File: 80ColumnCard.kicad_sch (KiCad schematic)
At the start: 37 parts, among them J1 Apple II Expansion Bus, J2 VIDEO & LIGHT PEN, Q1 2N3904, U1 74LS86, U14 74LS157, U15 74LS157, U16 74LS157, U18 74LS273, U19 MC6845, U2 74LS02, U21 74LS166, U22 74LS175, U23 74LS161, U3 2758{slash}16{slash}32, U4 74LS04, U5 74LS245, U6 74LS00, U7 4013, U8 4013, U9 74LS139, X6 CHAR INV, X7 SCREEN INV, Y1 17.430 MHZ

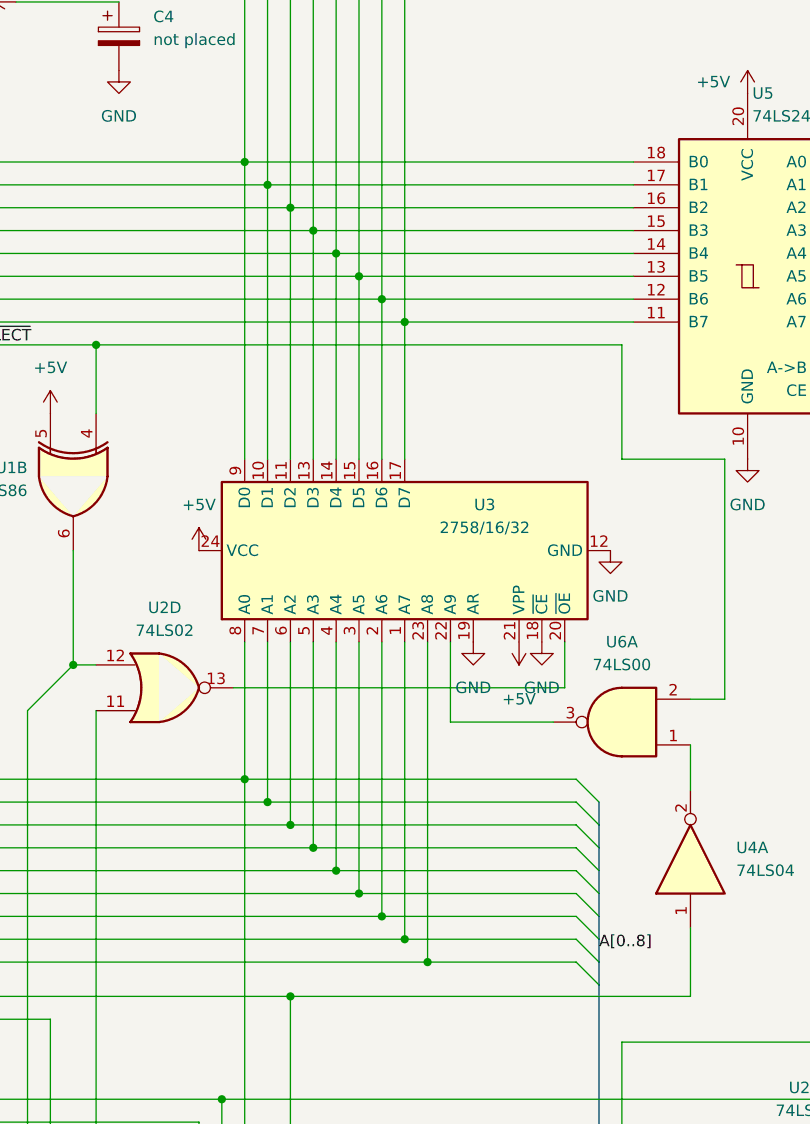
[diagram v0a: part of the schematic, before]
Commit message: updates
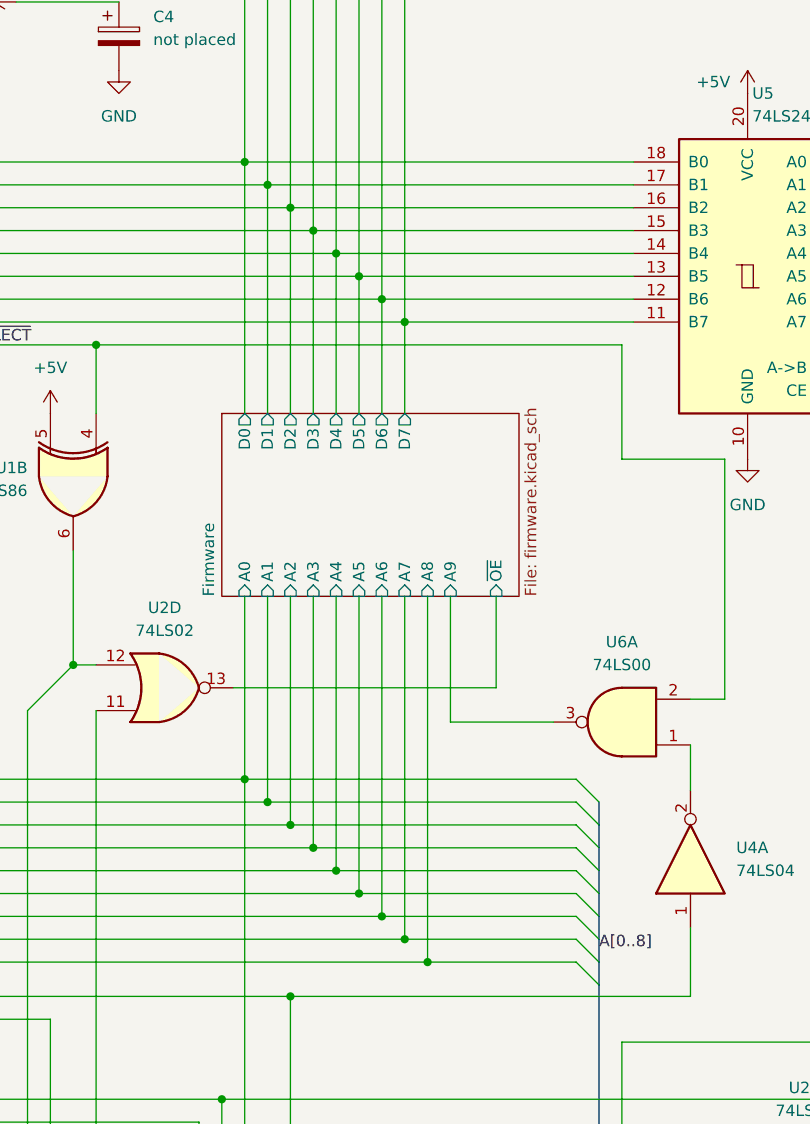
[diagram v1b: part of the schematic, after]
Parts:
- removed U3: 2758/16/32, MyPackages:DIP-24_W15.24mm, symbol ambassador:2758
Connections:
- net Firmware/A9: now reaches U6.3
- net Firmware/~{OE}: now reaches U2.13
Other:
- added sheet Firmware (firmware.kicad_sch)
